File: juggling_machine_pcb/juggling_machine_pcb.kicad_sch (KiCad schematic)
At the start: 16 parts, among them J1 Conn_01x08, J10 Screw_Terminal_01x04, J11 Screw_Terminal_01x04, J2 Conn_01x08, J3 Conn_01x08, J4 Conn_01x08, J5 servo 1, J6 servo 2, J7 24v input, J8 5v input, J9 24v out for input to buck

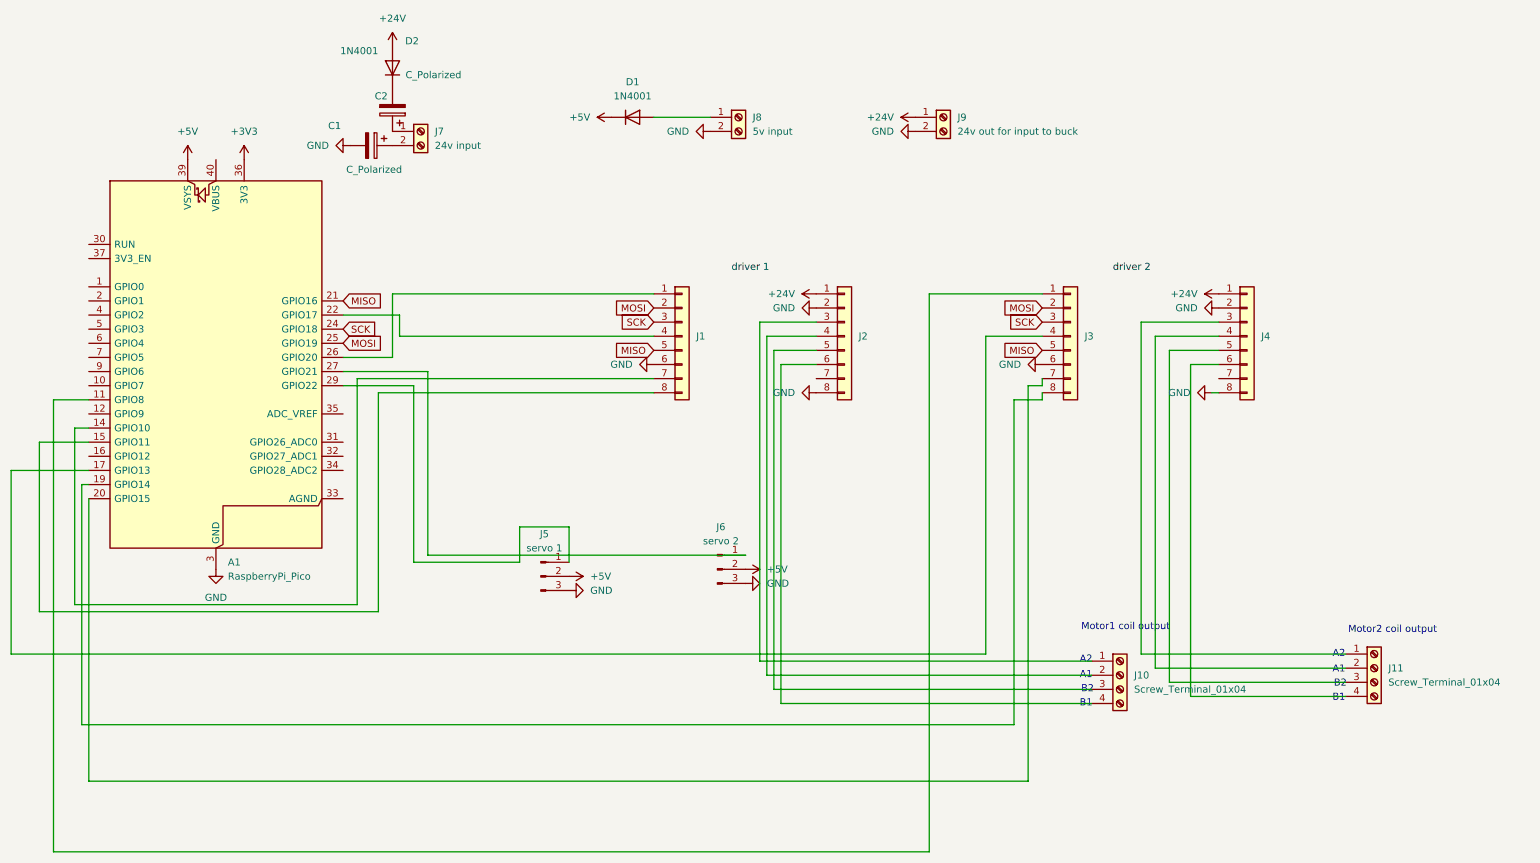
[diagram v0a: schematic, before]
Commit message: added new BOM, plus updated pcb
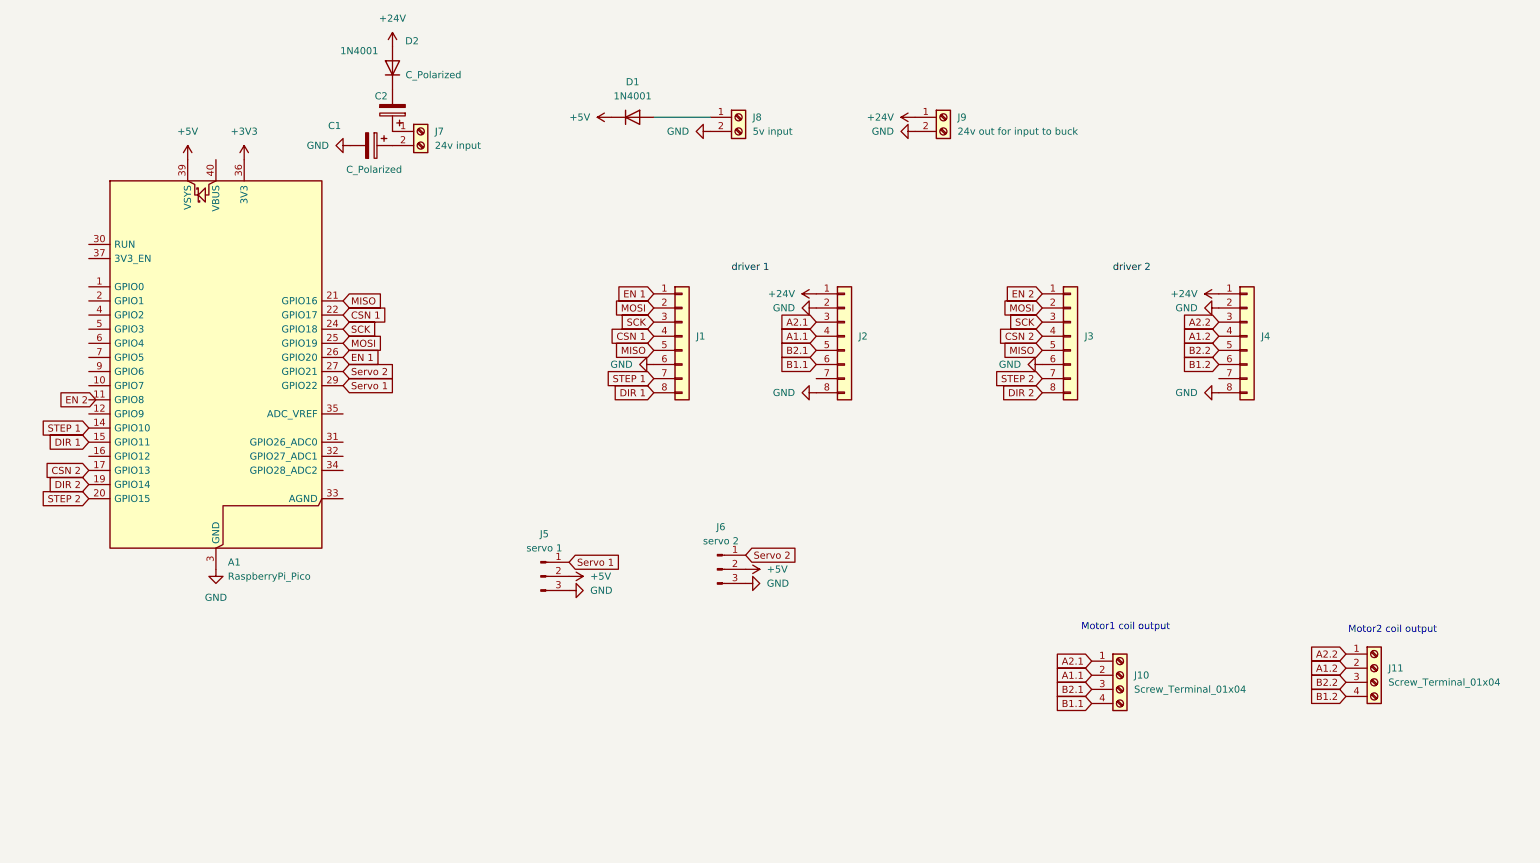
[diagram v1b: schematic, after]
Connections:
- net at A1.11 (GPIO8): no longer J3.1 (Pin_1)
- net CSN 2: now reaches A1.17 (GPIO13), J3.4 (Pin_4)
- net STEP 2: now reaches A1.20 (GPIO15), J3.7 (Pin_7)
- net DIR 2: now reaches A1.19 (GPIO14), J3.8 (Pin_8)
- net Servo 2: now reaches A1.27 (GPIO21), J6.1 (Pin_1)
- net STEP 1: now reaches A1.14 (GPIO10), J1.7 (Pin_7)
- net DIR 1: now reaches A1.15 (GPIO11), J1.8 (Pin_8)
- net CSN 1: now reaches A1.22 (GPIO17), J1.4 (Pin_4)
- net EN 1: now reaches A1.26 (GPIO20), J1.1 (Pin_1)
- net Servo 1: now reaches A1.29 (GPIO22), J5.1 (Pin_1)
- net A2.2: now reaches J11.1 (Pin_1), J4.3 (Pin_3)
- net A1.2: now reaches J11.2 (Pin_2), J4.4 (Pin_4)
- net B2.2: now reaches J11.3 (Pin_3), J4.5 (Pin_5)
- net B1.2: now reaches J11.4 (Pin_4), J4.6 (Pin_6)
- net A2.1: now reaches J10.1 (Pin_1), J2.3 (Pin_3)
- net A1.1: now reaches J10.2 (Pin_2), J2.4 (Pin_4)
- net B2.1: now reaches J10.3 (Pin_3), J2.5 (Pin_5)
- net B1.1: now reaches J10.4 (Pin_4), J2.6 (Pin_6)
- new net EN 2: J3.1 (Pin_1)
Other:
- note removed: "A1"
- note removed: "A2"
- note removed: "B1"
- note removed: "B2"
